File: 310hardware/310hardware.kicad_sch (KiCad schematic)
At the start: 3 parts, among them M1 Motor_DC, M2 Motor_DC

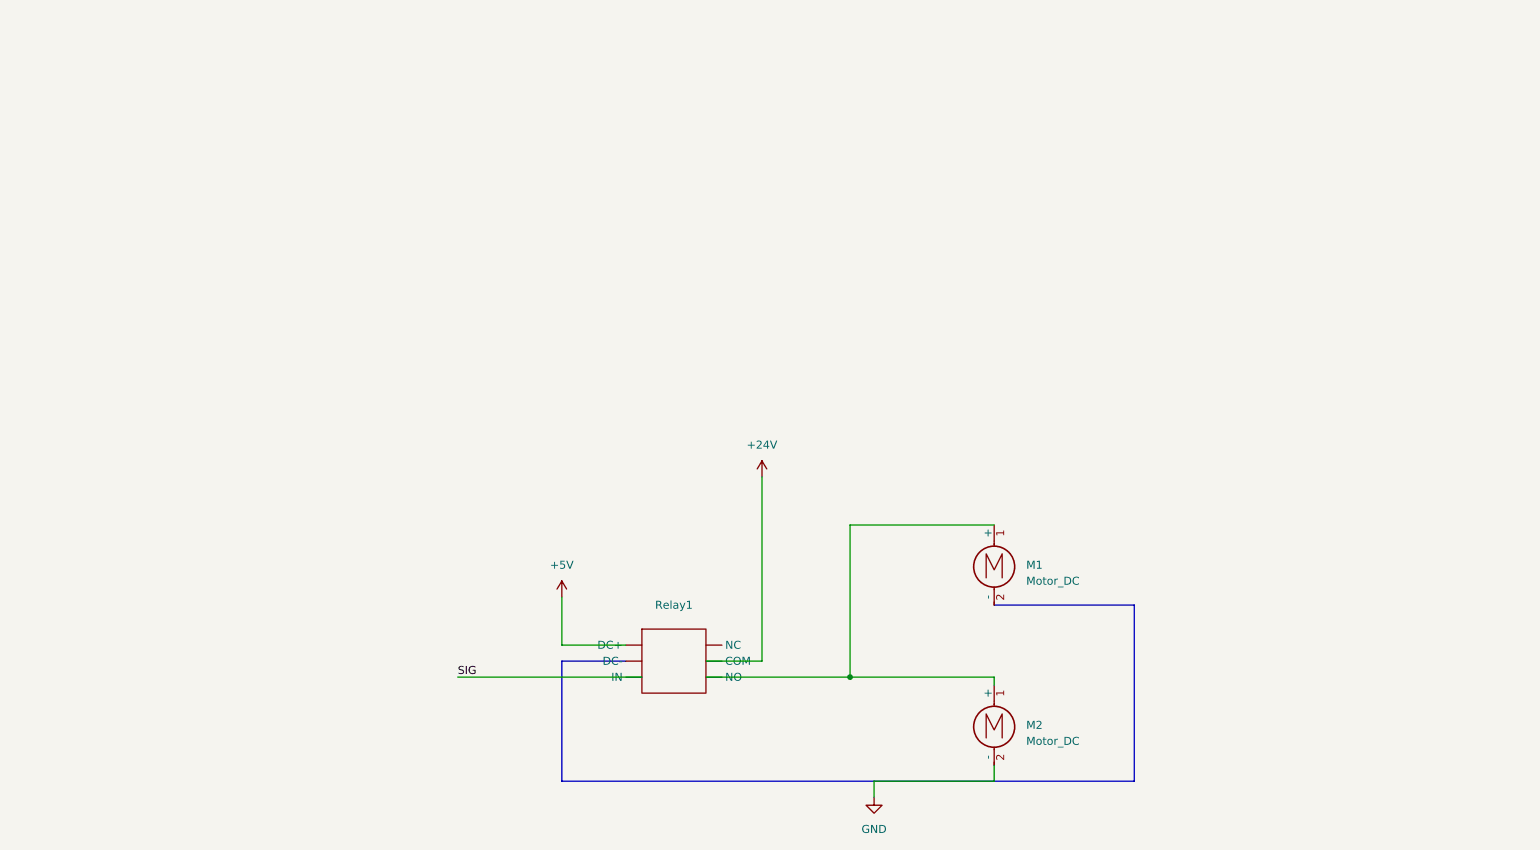
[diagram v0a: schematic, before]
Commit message: Final commit
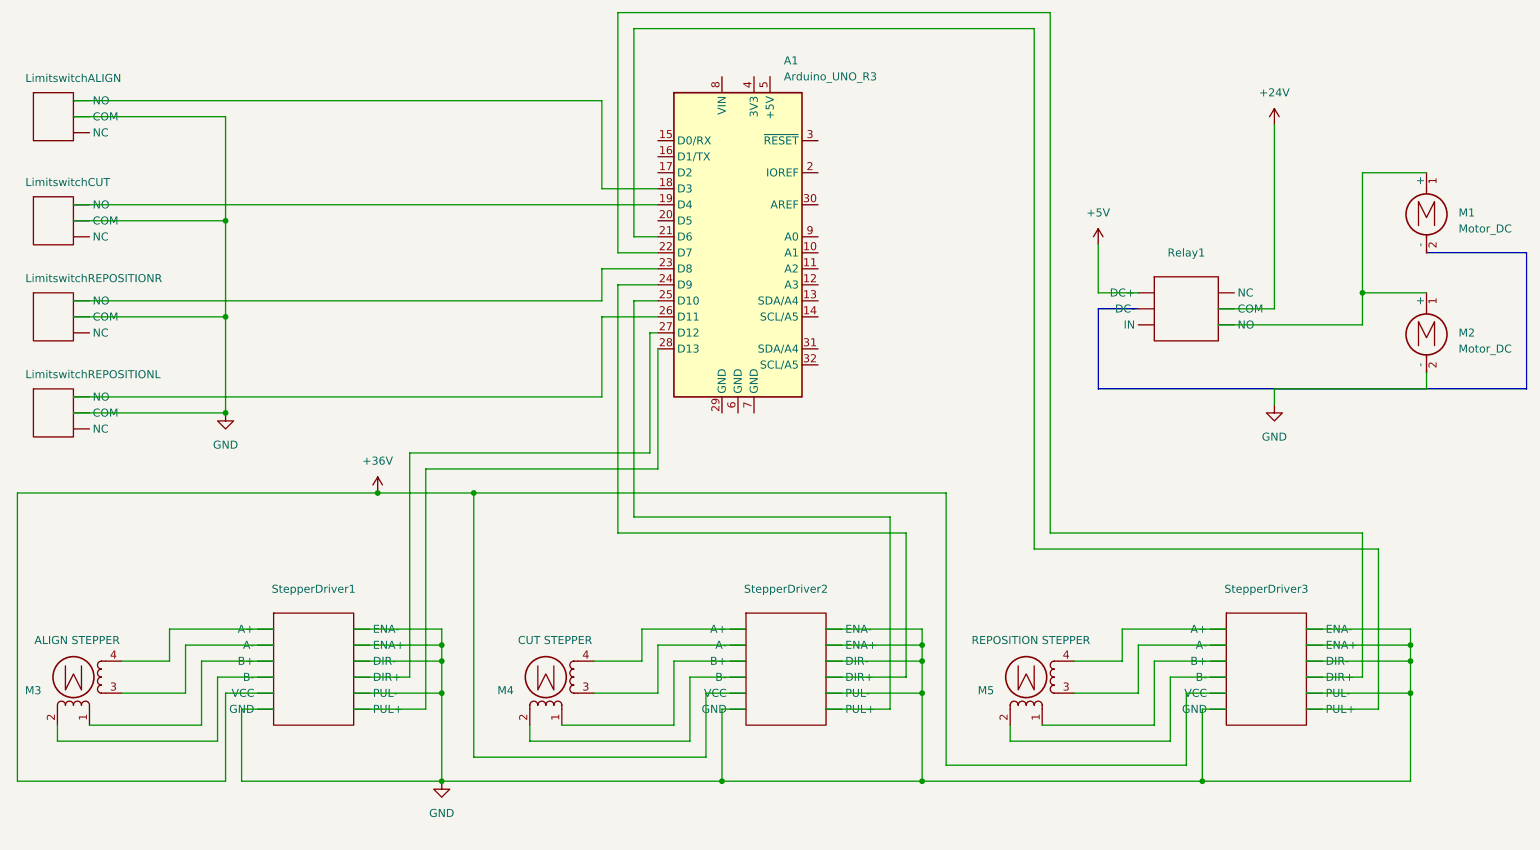
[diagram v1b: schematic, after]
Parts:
- added A1: Arduino_UNO_R3, Module:Arduino_UNO_R3, symbol MCU_Module:Arduino_UNO_R3
- added LimitswitchALIGN, LimitswitchCUT, LimitswitchREPOSITIONL, LimitswitchREPOSITIONR: ~, symbol 310hardwarelib:LImitswitch
- added M3: ALIGN STEPPER, symbol Motor:Stepper_Motor_bipolar
- added M4: CUT STEPPER, symbol Motor:Stepper_Motor_bipolar
- added M5: REPOSITION STEPPER, symbol Motor:Stepper_Motor_bipolar
- added StepperDriver1, StepperDriver2, StepperDriver3: ~, symbol 310hardwarelib:MicroStepperDriver
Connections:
- net SIG is gone; now on net +24V: Relay1. (NO)
- net GND: now also LimitswitchALIGN. (NO), LimitswitchCUT. (NO), LimitswitchREPOSITIONL. (NO), LimitswitchREPOSITIONR. (NO), StepperDriver1. (VCC), StepperDriver2. (VCC), StepperDriver3. (VCC)
- new net: M3.1, StepperDriver1. (VCC)
- new net: M3.2 (-), StepperDriver1. (VCC)
- new net: M3.3, StepperDriver1. (VCC)
- new net: M3.4, StepperDriver1. (VCC)
- new net: A1.27 (D12), StepperDriver1. (VCC)
- new net: A1.28 (D13), StepperDriver1. (VCC)
- new net: M4.1, StepperDriver2. (VCC)
- new net: M4.2 (-), StepperDriver2. (VCC)
- new net: M4.3, StepperDriver2. (VCC)
- new net: M4.4, StepperDriver2. (VCC)
- new net: A1.19 (D4), LimitswitchCUT. (NO)
- new net: M5.1, StepperDriver3. (VCC)
- new net: M5.2 (-), StepperDriver3. (VCC)
- new net: M5.3, StepperDriver3. (VCC)
- new net: M5.4, StepperDriver3. (VCC)
- new net: A1.26 (D11), LimitswitchREPOSITIONL. (NO)
- new net: A1.23 (D8), LimitswitchREPOSITIONR. (NO)
- new net: A1.18 (D3), LimitswitchALIGN. (NO)
- new net: A1.21 (D6), StepperDriver3. (VCC)
- new net: A1.22 (D7), StepperDriver3. (VCC)
- new net: A1.24 (D9), StepperDriver2. (VCC)
- new net: A1.25 (D10), StepperDriver2. (VCC)
- new net +36V: StepperDriver1. (VCC), StepperDriver2. (VCC), StepperDriver3. (VCC)
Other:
- moved on the sheet: M1, M2, Relay1
